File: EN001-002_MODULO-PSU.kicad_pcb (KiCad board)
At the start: 2 copper layers, 70 x 50 mm, 91 parts, among them J1 2x5P 2.54mm, J2 Conn_01x02, J3 Barrel_Jack_Switch, J5 1x3P 2mm, J6 Conn_01x04, Q1 AO3401, Q10 AO3401, Q11 KY6802, Q13 MMBT2222A, Q2 AO3401, Q3 KY6802, Q4 AO3401, Q5 AO3401, Q6 KY6802, Q7 KY6802, Q8 KY6802, Q9 AO3401, SW1 SK12D07VG3, SW2 TC-6615-7-260G, U1 AZ34063UMTR-G1, U2 74HC132D,653, U3 TP4056

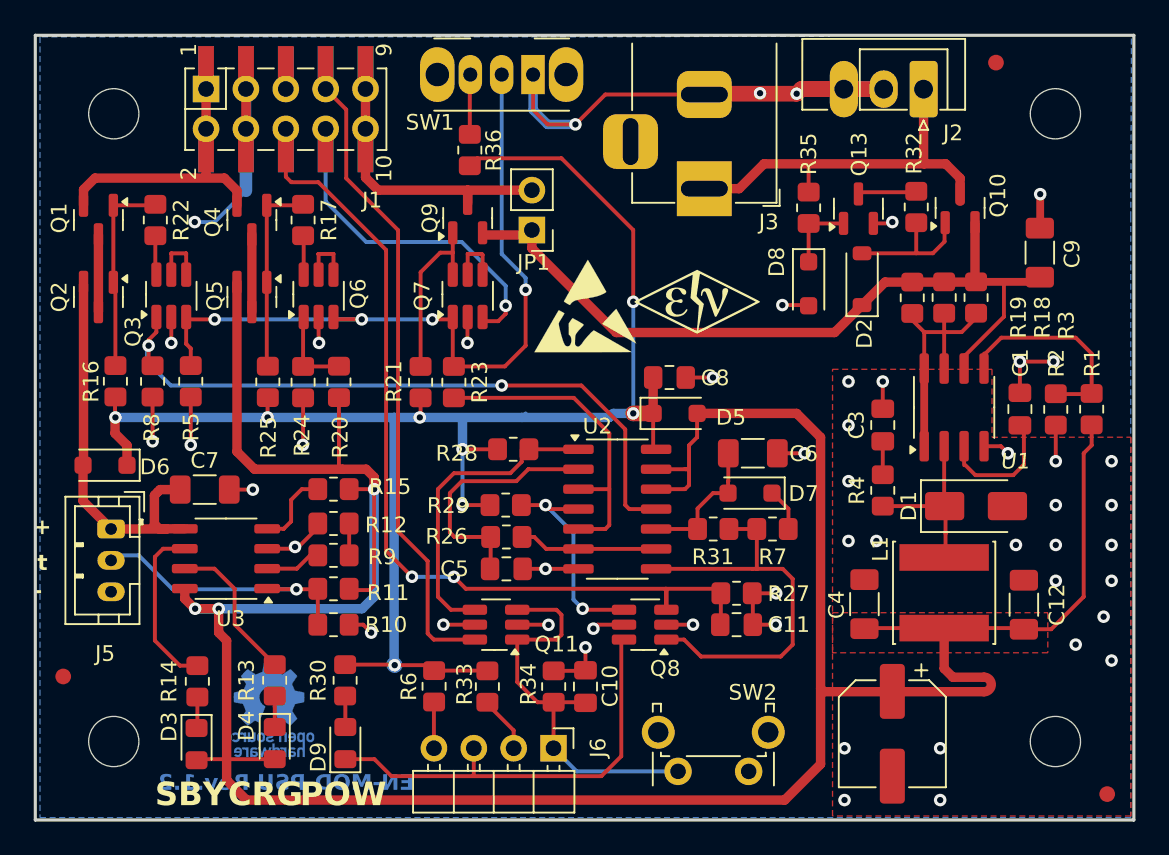
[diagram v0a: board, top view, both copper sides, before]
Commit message: kicad 8.0.5
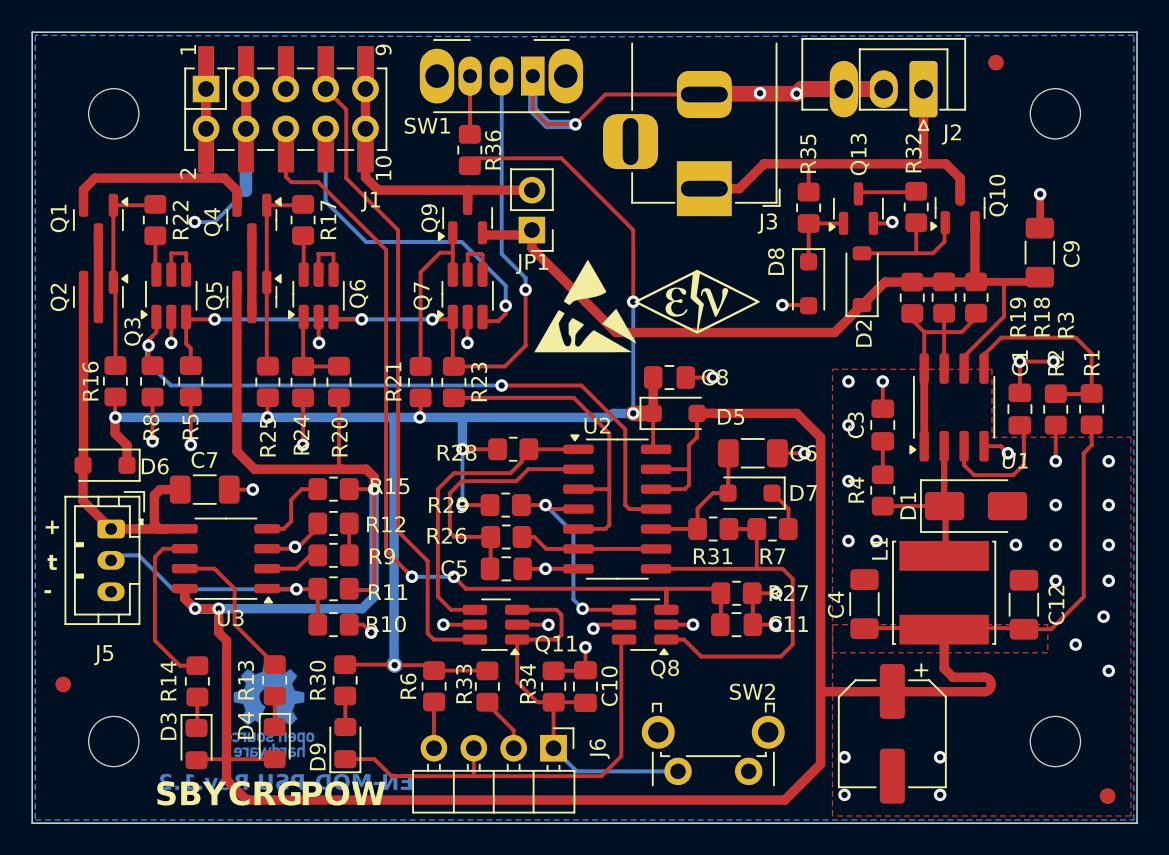
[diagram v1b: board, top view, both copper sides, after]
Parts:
- moved FID1 0.51 mm to (127.6, 78.0)
- moved FID2 0.13 mm to (194.1, 85.1)
- moved SW1 0.10 mm to (157.5, 39.2)
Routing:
- net /VOUT: track 17.8 -> 20.3 mm
- net /VINS: track 50.7 -> 48.8 mm
- net /VLOGIC: track 104.9 -> 103.7 mm
- net GND: track 103.0 -> 101.8 mm
- net Net-(U1-DRV): track 16.0 -> 15.3 mm
- net /5V#: track 43.0 -> 42.4 mm
- net /DRIVE: track 48.3 -> 47.8 mm
- net /VPOW: track 19.4 -> 18.8 mm
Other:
- board size 70 x 50 mm -> 70.4 x 50.4 mm
- rule pad_to_mask_clearance: 0 -> 0.1
